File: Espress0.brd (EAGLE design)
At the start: 36.8 x 39.4 mm, 41 parts, among them CN1 4U#20329, Q2 reset, U1 AP2112K-3.3, U2 2MB Flash, U3 MCP73831T-2ACI/OT

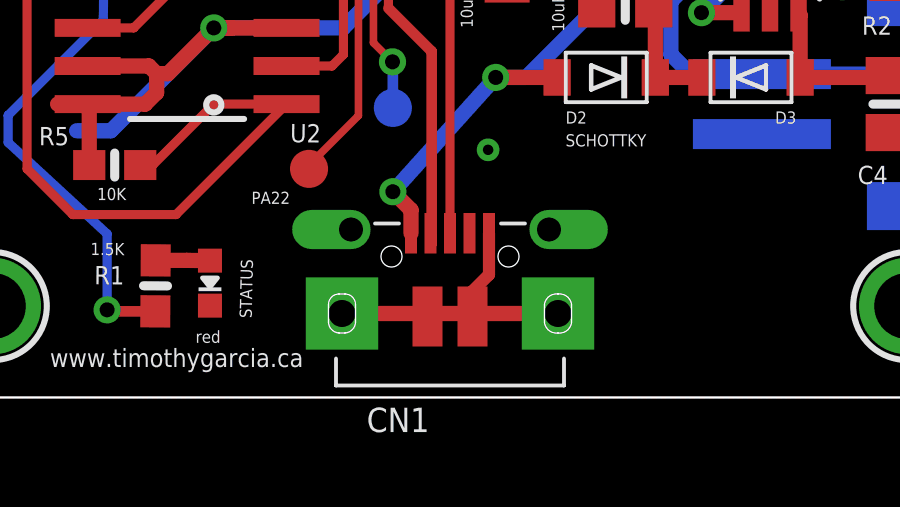
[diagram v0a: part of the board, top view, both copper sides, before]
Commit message: Add files via upload
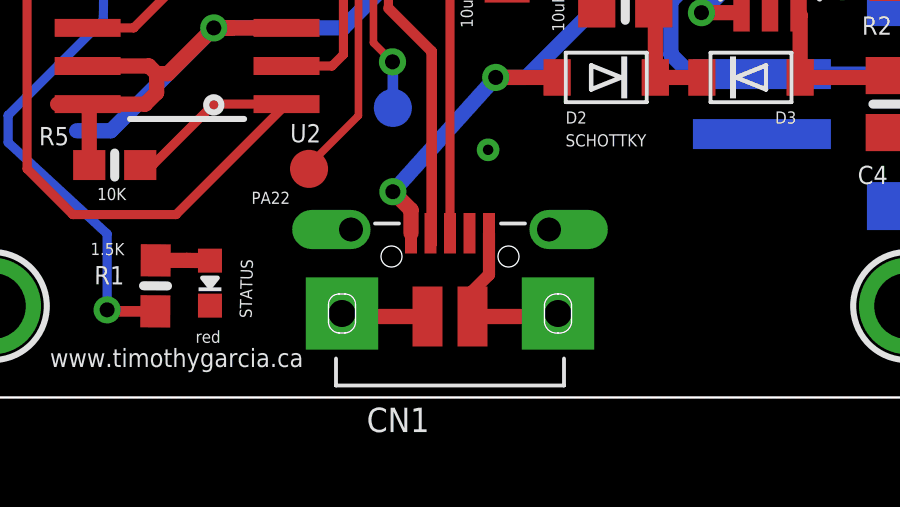
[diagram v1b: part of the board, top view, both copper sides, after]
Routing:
- net GND: track 11.7 -> 10.4 mm
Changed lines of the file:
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@@
 <wire x1="19.265" y1="2.799" x2="19.165" y2="2.699" width="0.508" layer="1"/>
 <wire x1="14.815" y1="2.799" x2="14.815" y2="2.667" width="0.508" layer="1"/>
-<wire x1="22.015" y1="2.799" x2="14.815" y2="2.799" width="0.508" layer="1"/>
-<wire x1="19.715" y1="4.094" x2="22.015" y2="2.799" width="0" layer="19" extent="1-1"/>
+<wire x1="22.015" y1="2.799" x2="22.015" y2="2.699" width="0.508" layer="1"/>
+<wire x1="22.015" y1="2.699" x2="19.165" y2="2.699" width="0.508" layer="1"/>
+<wire x1="14.815" y1="2.799" x2="14.815" y2="2.699" width="0.508" layer="1"/>
+<wire x1="14.815" y1="2.699" x2="17.665" y2="2.699" width="0.508" layer="1"/>
 </signal>
 <signal name="D+">
